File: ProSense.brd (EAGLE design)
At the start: 16.3 x 37.7 mm, 24 parts

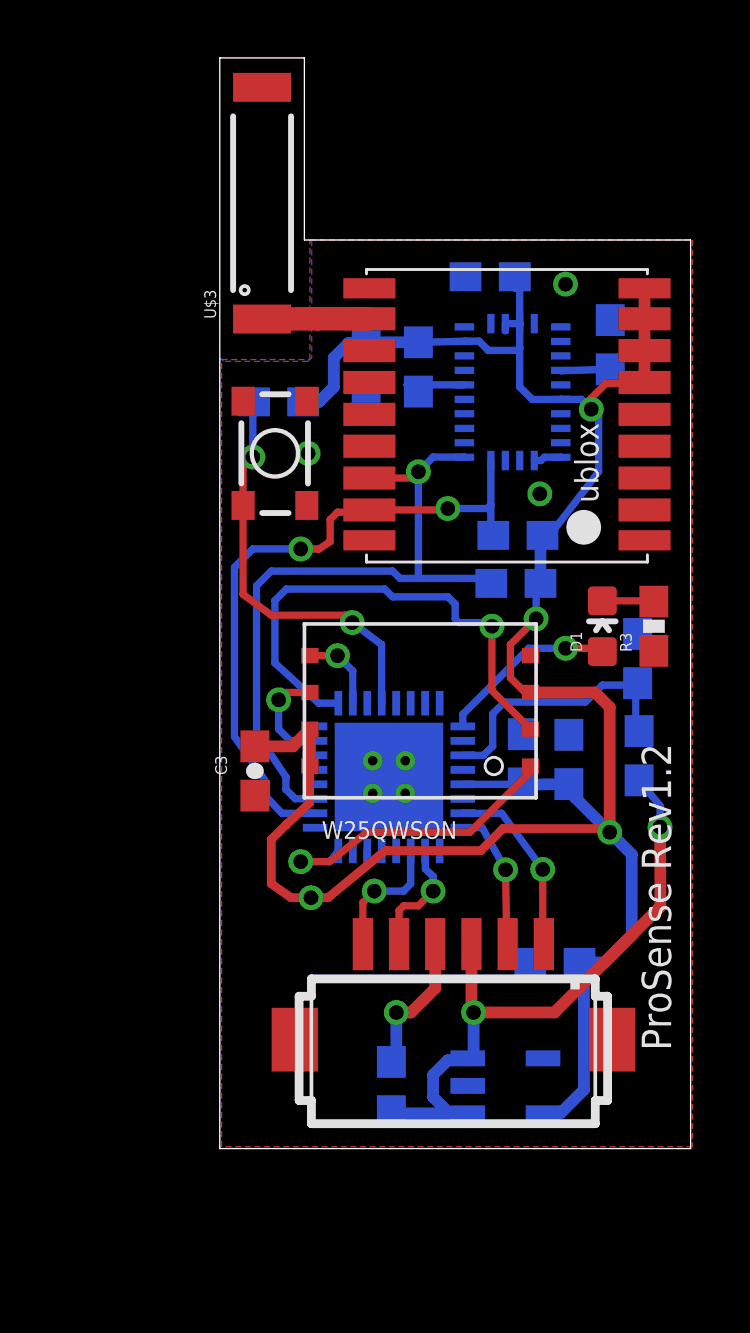
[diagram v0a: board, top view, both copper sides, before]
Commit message: Squash
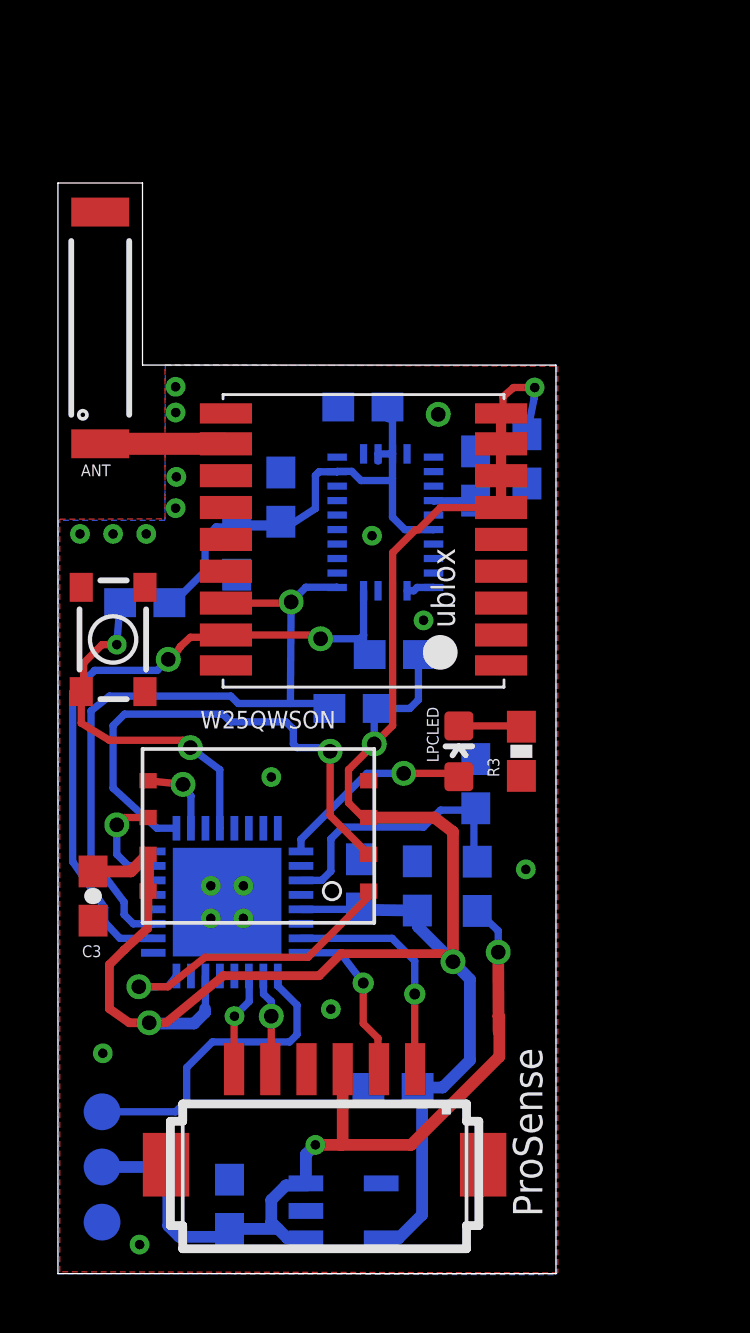
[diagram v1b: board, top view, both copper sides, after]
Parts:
- removed D1: (no value), SparkFun-LED:LED-0603
- removed U$3: ANTENNA2SMD3, SparkFun-RF:ANTENNA-CHIP4
- added ANT: ANTENNA2SMD3, SparkFun-RF:ANTENNA-CHIP4
- added C4: .1uF, SparkFun-Passives:0603-CAP
- added LPCLED: (no value), SparkFun-LED:LED-0603
- added U$4: CON, Matts-Parts:COPPER-PAD
- moved S2 8.52 mm to (1.91, 21.9)
- moved R4 8.33 mm to (3.00, 23.2)
- moved C5 7.75 mm to (6.17, 25.0)
- moved R1 7.18 mm to (14.5, 13.4)
- moved R2 7.06 mm to (14.4, 16.9)
- moved R8 7.06 mm to (10.2, 19.5)
- moved W25QWSON 7.06 mm to (6.92, 15.1)
- moved C8 7.06 mm to (10.4, 13.5)
- moved MIC5205 7.06 mm to (9.86, 2.17)
- moved C15 7.06 mm to (11.6, 6.43)
- moved C3 7.06 mm to (1.21, 13.0)
- moved MCU 7.06 mm to (5.84, 12.8)
- moved C14 6.91 mm to (5.92, 2.39)
- moved C7 6.82 mm to (12.4, 13.4)
- moved U$2 6.57 mm to (10.4, 25.4)
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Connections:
- new net SIG: MCU.1, U$4.SIG
- net GND: now also C4.1, U$4.GND
- net LED: now also LPCLED.A; no longer D1.A
- net N$1: now also ANT.SIG; no longer U$3.SIG
- net N$5: now also LPCLED.C; no longer D1.C
- net VCC: now also C4.2
- net VIN: now also U$4.VLED
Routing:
- net VCC: track 83.3 -> 95.0 mm
- net SIG: track 0.00 -> 10.8 mm
- net GND: track 8.63 -> 0.96 mm, vias 4 -> 15
- net VIN: track 23.1 -> 29.4 mm
- net BTN: track 14.2 -> 12.5 mm
- net LPC_RX: track 6.34 -> 7.99 mm
- net SCL: track 23.0 -> 24.1 mm
- net ISP: track 4.49 -> 3.44 mm
- net LPC_TX: track 4.91 -> 5.87 mm
- net RESET: track 4.12 -> 3.35 mm
- net LED: track 6.23 -> 6.86 mm
- net N$1: track 3.71 -> 4.34 mm
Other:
- board size 16.3 x 37.7 mm -> 17.2 x 37.7 mm
- board text added: "ProSense"
- board text removed: "ProSense Rev1.2"
